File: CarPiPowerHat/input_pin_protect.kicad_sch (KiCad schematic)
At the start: 7 parts

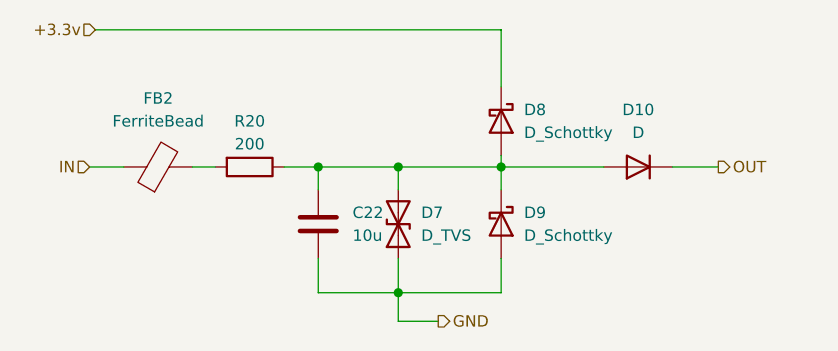
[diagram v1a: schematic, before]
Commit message: Finished Layout
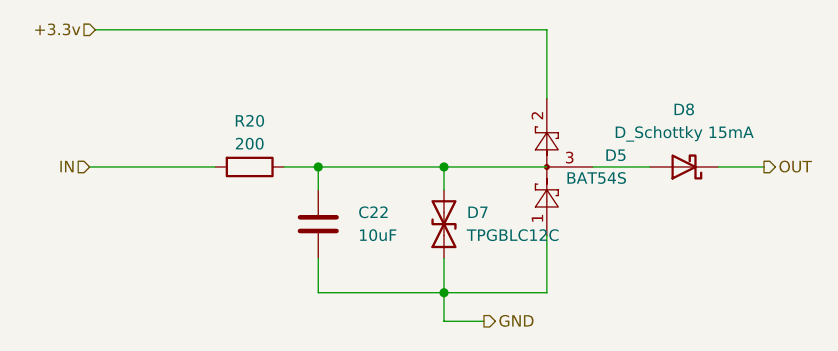
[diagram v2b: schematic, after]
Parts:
- removed D10: D, Diode_SMD:D_SOD-123F, symbol Device:D
- removed D9: D_Schottky, Diode_SMD:D_SOD-123, symbol Device:D_Schottky
- removed FB2: FerriteBead, Resistor_SMD:R_0805_2012Metric, symbol Device:FerriteBead
- added D5: BAT54S, Package_TO_SOT_SMD:SOT-23, symbol Diode:BAT54S
- C22: value 10u -> 10uF; footprint Resistor_SMD:R_0603_1608Metric -> Capacitor_SMD:C_0603_1608Metric
- D7: value D_TVS -> TPGBLC12C; footprint Diode_SMD:D_0603_1608Metric -> Diode_SMD:D_SOD-323; LCSC (none) -> C587149
- D8: value D_Schottky -> D_Schottky 15mA; footprint Diode_SMD:D_SOD-123 -> Diode_SMD:D_SOD-323; LCSC C8598 -> C508253
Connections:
- net +3.3v: now also D5.2; no longer D8.1 (K)
- net GND: now also D5.1
- net IN: now also R20.2
- net OUT: now also D8.1 (K)
- net at C22.1, D7.2 (A2), R20.1: no longer D8.2 (A)
- new net: D5.3, D8.2 (A)
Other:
- moved on the sheet: D7
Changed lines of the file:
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@@
   (paper "A4")
   (junction (at 129.54 80.01) (diameter 1.016) (color 0 0 0 0))
-  (junction (at 138.43 80.01) (diameter 1.016) (color 0 0 0 0))
-  (junction (at 138.43 93.98) (diameter 1.016) (color 0 0 0 0))
-  (junction (at 149.86 80.01) (diameter 1.016) (color 0 0 0 0))
-  (wire (pts (xy 104.14 80.01) (xy 107.95 80.01))
+  (junction (at 143.51 80.01) (diameter 1.016) (color 0 0 0 0))
+  (junction (at 143.51 93.98) (diameter 1.016) (color 0 0 0 0))
+  (wire (pts (xy 104.14 80.01) (xy 118.11 80.01))
     (stroke (width 0) (type solid) (color 0 0 0 0))
   )
-  (wire (pts (xy 104.775 64.77) (xy 149.86 64.77))
-    (stroke (width 0) (type solid) (color 0 0 0 0))
-  )
-  (wire (pts (xy 115.57 80.01) (xy 118.11 80.01))
+  (wire (pts (xy 104.775 64.77) (xy 154.94 64.77))
     (stroke (width 0) (type solid) (color 0 0 0 0))
   )
@@
     (stroke (width 0) (type solid) (color 0 0 0 0))
   )
-  (wire (pts (xy 129.54 80.01) (xy 138.43 80.01))
+  (wire (pts (xy 129.54 80.01) (xy 143.51 80.01))
     (stroke (width 0) (type solid) (color 0 0 0 0))
   )
@@
     (stroke (width 0) (type solid) (color 0 0 0 0))
   )
-  (wire (pts (xy 129.54 93.98) (xy 138.43 93.98))
+  (wire (pts (xy 129.54 93.98) (xy 143.51 93.98))
     (stroke (width 0) (type solid) (color 0 0 0 0))
   )
-  (wire (pts (xy 138.43 80.01) (xy 149.86 80.01))
+  (wire (pts (xy 143.51 80.01) (xy 154.94 80.01))
     (stroke (width 0) (type solid) (color 0 0 0 0))
   )
-  (wire (pts (xy 138.43 82.55) (xy 138.43 80.01))
+  (wire (pts (xy 143.51 82.55) (xy 143.51 80.01))
     (stroke (width 0) (type solid) (color 0 0 0 0))
   )
-  (wire (pts (xy 138.43 93.98) (xy 138.43 90.17))
+  (wire (pts (xy 143.51 93.98) (xy 143.51 90.17))
     (stroke (width 0) (type solid) (color 0 0 0 0))
   )
-  (wire (pts (xy 138.43 93.98) (xy 138.43 97.155))
+  (wire (pts (xy 143.51 93.98) (xy 143.51 97.155))
     (stroke (width 0) (type solid) (color 0 0 0 0))
   )
-  (wire (pts (xy 138.43 97.155) (xy 142.875 97.155))
+  (wire (pts (xy 143.51 97.155) (xy 147.955 97.155))
     (stroke (width 0) (type solid) (color 0 0 0 0))
   )
-  (wire (pts (xy 149.86 64.77) (xy 149.86 71.12))
+  (wire (pts (xy 154.94 64.77) (xy 154.94 72.39))
     (stroke (width 0) (type solid) (color 0 0 0 0))
   )
-  (wire (pts (xy 149.86 78.74) (xy 149.86 80.01))
+  (wire (pts (xy 154.94 87.63) (xy 154.94 93.98))
     (stroke (width 0) (type solid) (color 0 0 0 0))
   )
-  (wire (pts (xy 149.86 80.01) (xy 149.86 82.55))
+  (wire (pts (xy 154.94 93.98) (xy 143.51 93.98))
     (stroke (width 0) (type solid) (color 0 0 0 0))
   )
-  (wire (pts (xy 149.86 80.01) (xy 161.29 80.01))
+  (wire (pts (xy 160.02 80.01) (xy 166.37 80.01))
     (stroke (width 0) (type solid) (color 0 0 0 0))
   )
-  (wire (pts (xy 149.86 90.17) (xy 149.86 93.98))
-    (stroke (width 0) (type solid) (color 0 0 0 0))
-  )
-  (wire (pts (xy 149.86 93.98) (xy 138.43 93.98))
-    (stroke (width 0) (type solid) (color 0 0 0 0))
-  )
-  (wire (pts (xy 168.91 80.01) (xy 173.99 80.01))
+  (wire (pts (xy 173.99 80.01) (xy 179.07 80.01))
     (stroke (width 0) (type solid) (color 0 0 0 0))
   )
@@
     (effects (font (size 1.27 1.27)) (justify right))
   )
-  (hierarchical_label "GND" (shape output) (at 142.875 97.155 0)
+  (hierarchical_label "GND" (shape output) (at 147.955 97.155 0)
     (effects (font (size 1.27 1.27)) (justify left))
   )
-  (hierarchical_label "OUT" (shape output) (at 173.99 80.01 0)
+  (hierarchical_label "OUT" (shape output) (at 179.07 80.01 0)
     (effects (font (size 1.27 1.27)) (justify left))
   )
@@
     (pin "2")
   )
-  (symbol (lib_id "Device:D_TVS") (at 138.43 86.36 90)
+  (symbol (lib_id "Device:D_TVS") (at 143.51 86.36 90)
     (in_bom yes) (on_board yes)
-    (property "Reference" "D7" (id 0) (at 140.97 85.09 90)
+    (property "Reference" "D7" (id 0) (at 146.05 85.09 90)
       (effects (font (size 1.27 1.27)) (justify right))
     )
-    (property "Value" "D_TVS" (id 1) (at 140.97 87.63 90)
+    (property "Value" "TPGBLC12C" (id 1) (at 146.05 87.63 90)
       (effects (font (size 1.27 1.27)) (justify right))
     )
-    (property "Footprint" "Diode_SMD:D_0603_1608Metric" (id 2) (at 138.43 86.36 0)
+    (property "Footprint" "Diode_SMD:D_SOD-323" (id 2) (at 143.51 86.36 0)
       (effects (font (size 1.27 1.27)) hide)
     )
-    (property "Datasheet" "~" (id 3) (at 138.43 86.36 0)
+    (property "Datasheet" "~" (id 3) (at 143.51 86.36 0)
+      (effects (font (size 1.27 1.27)) hide)
+    )
+    (property "LCSC" "C587149" (id 4) (at 143.51 86.36 90)
       (effects (font (size 1.27 1.27)) hide)
     )
@@
     (pin "2")
   )
-  (symbol (lib_id "Device:D_Schottky") (at 149.86 74.93 270)
-    (in_bom yes) (on_board yes)
-    (property "Reference" "D8" (id 0) (at 152.4 73.66 90)
-      (effects (font (size 1.27 1.27)) (justify left))
-    )
-    (property "Value" "D_Schottky" (id 1) (at 152.4 76.2 90)
-      (effects (font (size 1.27 1.27)) (justify left))
-    )
-    (property "Footprint" "Diode_SMD:D_SOD-123" (id 2) (at 149.86 74.93 0)
+  (symbol (lib_id "Device:D_Schottky") (at 170.18 80.01 180)
+    (in_bom yes) (on_board yes) (fields_autoplaced)
+    (property "Reference" "D8" (id 0) (at 170.18 73.66 0))
+    (property "Value" "D_Schottky 15mA" (id 1) (at 170.18 76.2 0))
+    (property "Footprint" "Diode_SMD:D_SOD-323" (id 2) (at 170.18 80.01 0)
       (effects (font (size 1.27 1.27)) hide)
     )
-    (property "Datasheet" "~" (id 3) (at 149.86 74.93 0)
+    (property "Datasheet" "~" (id 3) (at 170.18 80.01 0)
       (effects (font (size 1.27 1.27)) hide)
     )
-    (property "LCSC" "C8598" (id 4) (at 149.86 74.93 90)
-      (effects (font (size 1.27 1.27)) hide)
-    )
-    (pin "1")
-    (pin "2")
-  )
-  (symbol (lib_id "Device:D_Schottky") (at 149.86 86.36 270)
-    (in_bom yes) (on_board yes)
-    (property "Reference" "D9" (id 0) (at 152.4 85.09 90)
-      (effects (font (size 1.27 1.27)) (justify left))
-    )
-    (property "Value" "D_Schottky" (id 1) (at 152.4 87.63 90)
-      (effects (font (size 1.27 1.27)) (justify left))
-    )
-    (property "Footprint" "Diode_SMD:D_SOD-123" (id 2) (at 149.86 86.36 0)
-      (effects (font (size 1.27 1.27)) hide)
-    )
-    (property "Datasheet" "~" (id 3) (at 149.86 86.36 0)
-      (effects (font (size 1.27 1.27)) hide)
-    )
-    (pin "1")
-    (pin "2")
-  )
-  (symbol (lib_id "Device:D") (at 165.1 80.01 180)
-    (in_bom yes) (on_board yes)
-    (property "Reference" "D10" (id 0) (at 165.1 73.66 0))
-    (property "Value" "D" (id 1) (at 165.1 76.2 0))
-    (property "Footprint" "Diode_SMD:D_SOD-123F" (id 2) (at 165.1 80.01 0)
-      (effects (font (size 1.27 1.27)) hide)
-    )
-    (property "Datasheet" "~" (id 3) (at 165.1 80.01 0)
-      (effects (font (size 1.27 1.27)) hide)
-    )
-    (property "LCSC" "C64898" (id 4) (at 165.1 80.01 0)
+    (property "LCSC" "C508253" (id 4) (at 170.18 80.01 0)
       (effects (font (size 1.27 1.27)) hide)
     )
@@
   (symbol (lib_id "Device:C") (at 129.54 86.36 0)
     (in_bom yes) (on_board yes)
-    (property "Reference" "C22" (id 0) (at 133.35 85.09 0)
+    (property "Reference" "C22" (id 0) (at 133.985 85.09 0)
       (effects (font (size 1.27 1.27)) (justify left))
     )
-    (property "Value" "10u" (id 1) (at 133.35 87.63 0)
+    (property "Value" "10uF" (id 1) (at 133.985 87.63 0)
       (effects (font (size 1.27 1.27)) (justify left))
     )
-    (property "Footprint" "Resistor_SMD:R_0603_1608Metric" (id 2) (at 130.5052 90.17 0)
+    (property "Footprint" "Capacitor_SMD:C_0603_1608Metric" (id 2) (at 130.5052 90.17 0)
       (effects (font (size 1.27 1.27)) hide)
     )
@@
     (pin "2")
   )
-  (symbol (lib_id "Device:FerriteBead") (at 111.76 80.01 90)
+  (symbol (lib_id "Diode:BAT54S") (at 154.94 80.01 90)
     (in_bom yes) (on_board yes)
-    (property "Reference" "FB2" (id 0) (at 111.76 72.39 90))
-    (property "Value" "FerriteBead" (id 1) (at 111.76 74.93 90))
-    (property "Footprint" "Resistor_SMD:R_0805_2012Metric" (id 2) (at 111.76 81.788 90)
-      (effects (font (size 1.27 1.27)) hide)
+    (property "Reference" "D5" (id 0) (at 163.83 78.7399 90)
+      (effects (font (size 1.27 1.27)) (justify left))
     )
-    (property "Datasheet" "~" (id 3) (at 111.76 80.01 0)
+    (property "Value" "BAT54S" (id 1) (at 163.83 81.2799 90)
+      (effects (font (size 1.27 1.27)) (justify left))
+    )
+    (property "Footprint" "Package_TO_SOT_SMD:SOT-23" (id 2) (at 151.765 78.105 0)
+      (effects (font (size 1.27 1.27)) (justify left) hide)
+    )
+    (property "Datasheet" "https://www.diodes.com/assets/Datasheets/ds11005.pdf" (id 3) (at 154.94 83.058 0)
       (effects (font (size 1.27 1.27)) hide)
     )
     (pin "1")
     (pin "2")
+    (pin "3")
   )
 )
